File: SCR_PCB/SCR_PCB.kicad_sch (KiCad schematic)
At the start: 4 parts, among them J1 RJ45, J2 Conn_01x03, U2 NA555D, U3 MAX941xSA

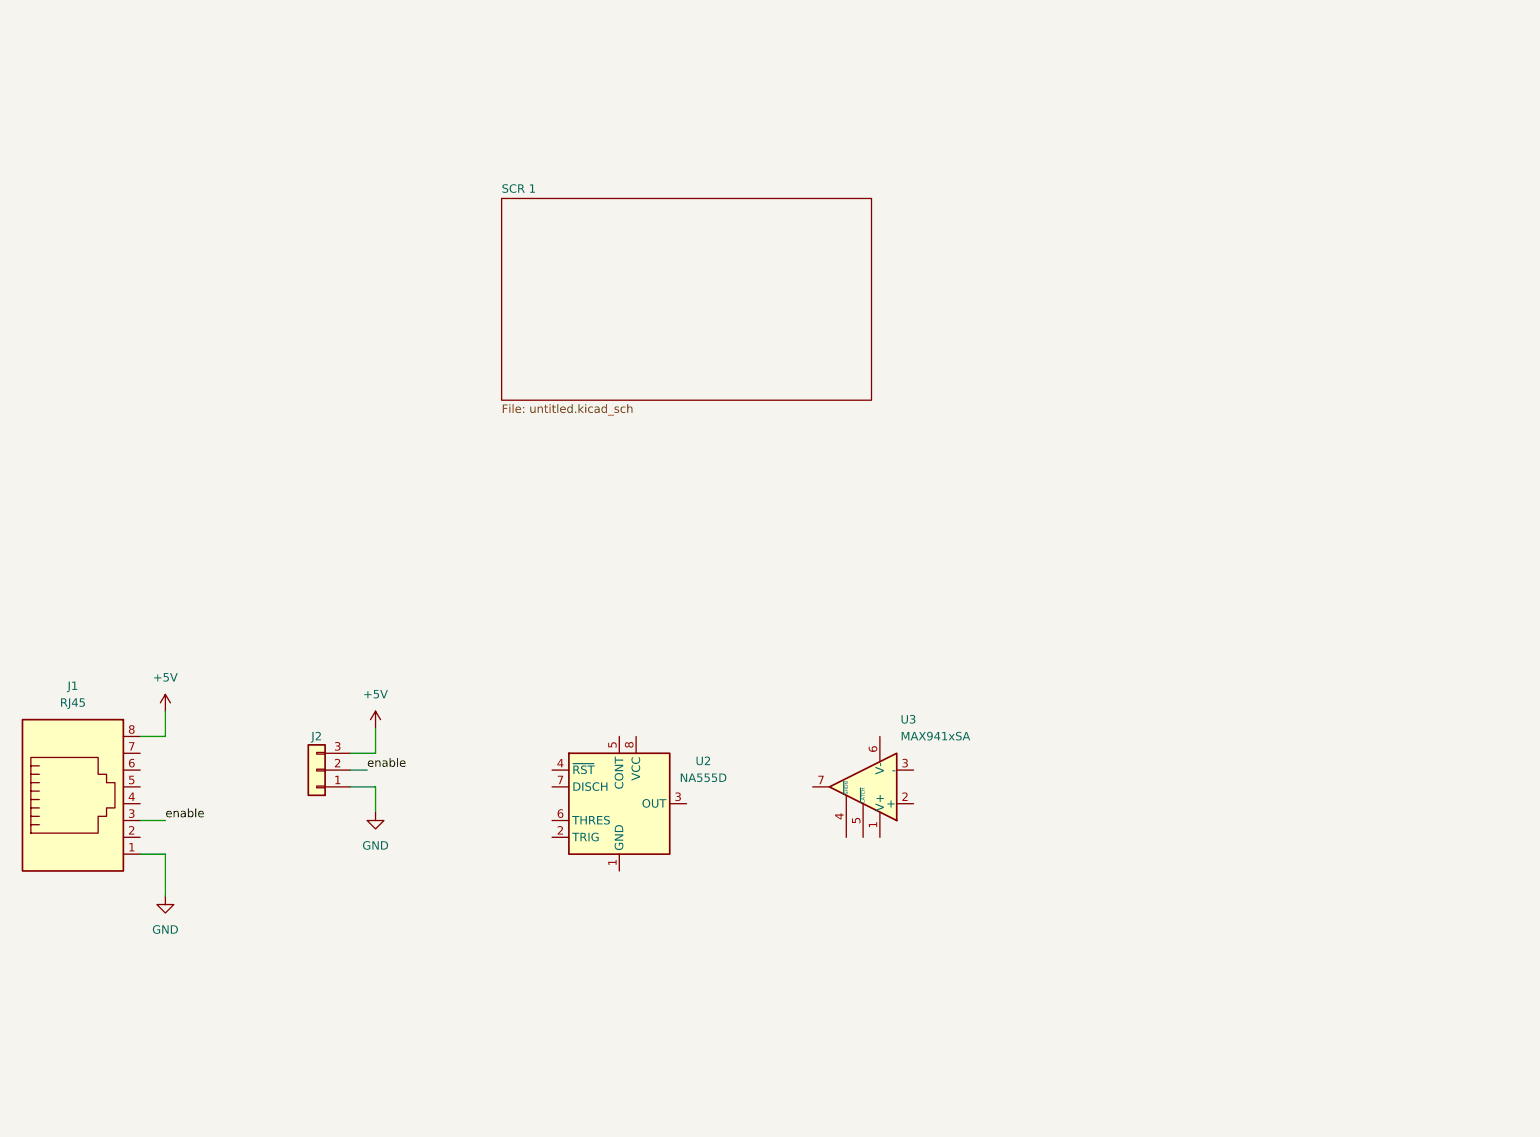
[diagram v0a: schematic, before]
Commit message: update SRC_PCB
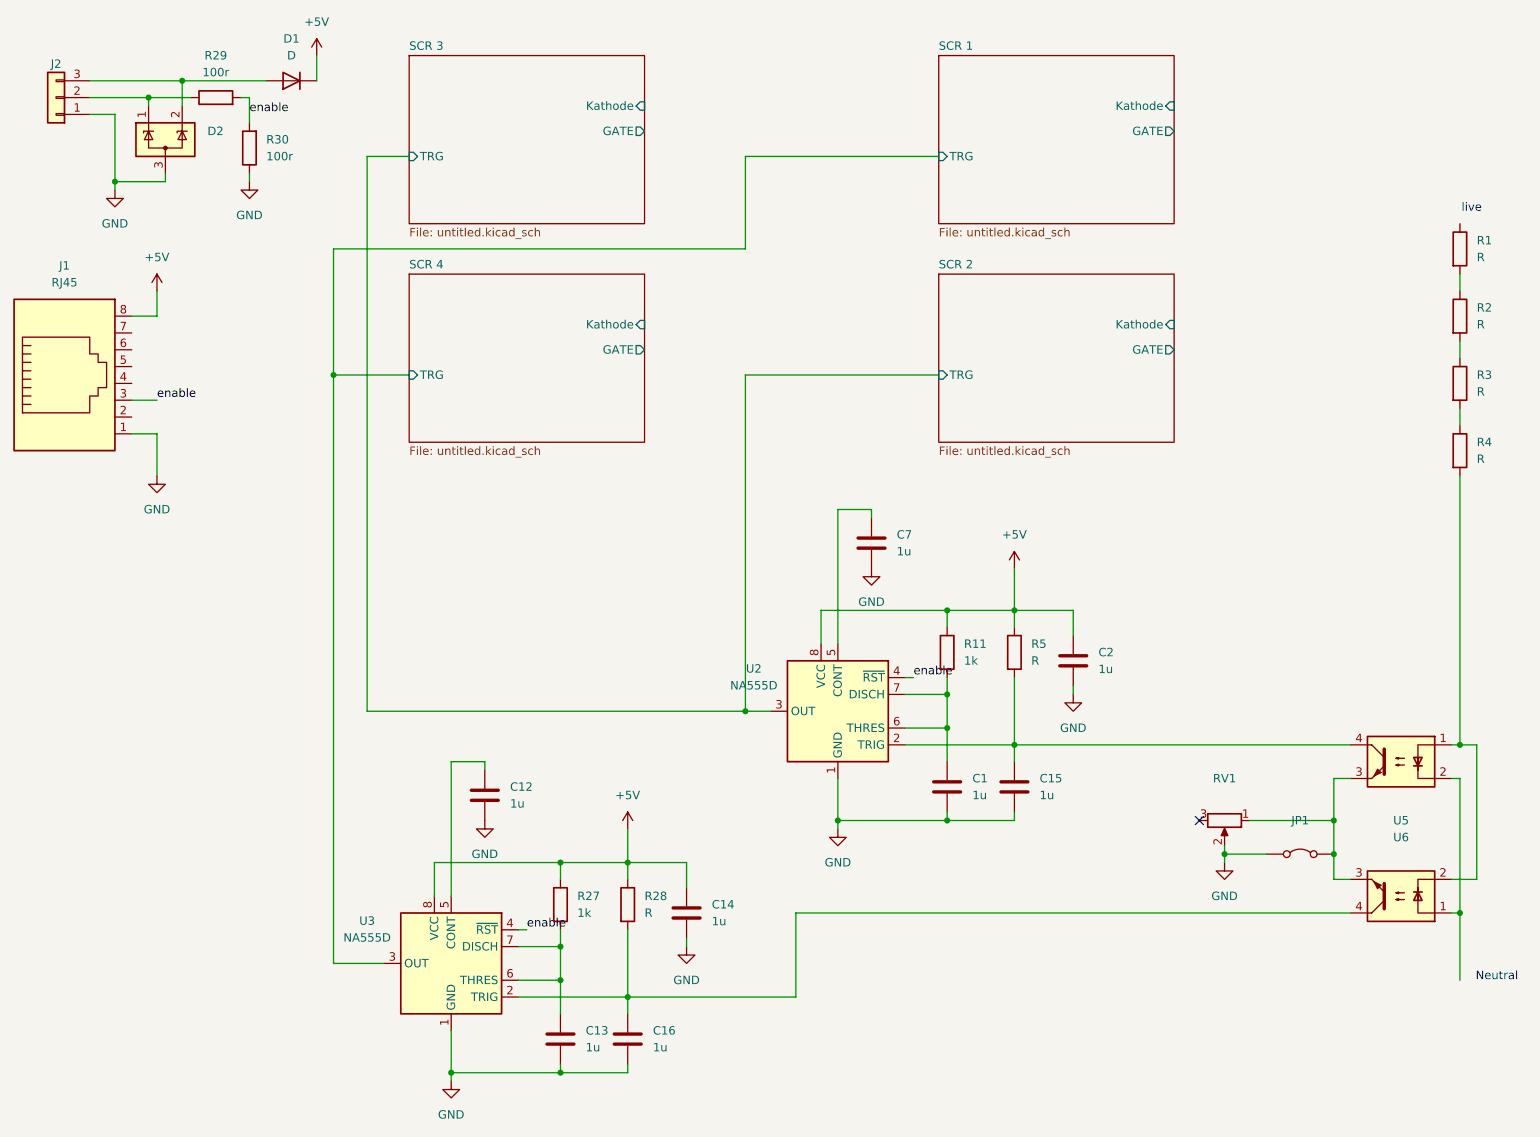
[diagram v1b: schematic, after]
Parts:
- removed U3: MAX941xSA, Package_SO:SOIC-8_3.9x4.9mm_P1.27mm, symbol Comparator:MAX941xSA
- added C1, C12, C13, C14, C15, C16, C2, C7: 1u, symbol Device:C
- added D1: D, symbol Device:D
- added D2: SP0502BAHT, Package_TO_SOT_SMD:SOT-23, symbol Power_Protection:SP0502BAHT
- added JP1: Jumper_2_Bridged, symbol Jumper:Jumper_2_Bridged
- added R1, R2, R28, R3, R4, R5: R, symbol Device:R
- added R11, R27: 1k, symbol Device:R
- added R29, R30: 100r, symbol Device:R
- added RV1: R_Potentiometer, symbol Device:R_Potentiometer
- added U3: NA555D, Package_SO:SOIC-8_3.9x4.9mm_P1.27mm, symbol Timer:NA555D
- added U5, U6: SFH617A-1, Package_DIP:DIP-4_W7.62mm, symbol Isolator:SFH617A-1
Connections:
- net +5V: now also U2.8 (VCC), C14.1, C2.1, D1.1 (K), R11.1, R27.1, R28.1, R5.1, U3.8 (VCC); no longer J2.3 (Pin_3)
- net GND: now also U2.1 (GND), C1.2, C12.2, C13.2, C14.2, C15.2, C16.2, C2.2, C7.2, D2.3 (A), JP1.1 (A), R30.1, RV1.2, U3.1 (GND)
- net enable: now also U2.4 (~{RST}), R29.2, R30.2, U3.4 (~{RST}); no longer J2.2 (Pin_2)
- net at U2.2 (TRIG): now also C15.1, R5.2, U5.4
- net SCR 2/TRG: now reaches U2.3 (OUT)
- net at U2.5 (CONT): now also C7.1
- net at U2.6 (THRES): now also U2.7 (DISCH), C1.1, R11.2
- new net: JP1.2 (B), RV1.1, U5.3, U6.3
- new net: D2.1 (K), J2.2 (Pin_2), R29.1
- new net: D1.2 (A), D2.2 (K), J2.3 (Pin_3)
- new net: R3.2, R4.1
- new net: R4.2, U5.1, U6.2
- new net: R1.2, R2.1
- new net: R2.2, R3.1
- new net: C12.1, U3.5 (CONT)
- new net: C16.1, R28.2, U3.2 (TRIG), U6.4
- new net: C13.1, R27.2, U3.6 (THRES), U3.7 (DISCH)
- new net: U5.2, U6.1
- new net SCR 1/TRG: U3.3 (OUT)
- no-connect marks 0 -> 1
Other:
- added sheet SCR 2 (untitled.kicad_sch)
- added sheet SCR 3 (untitled.kicad_sch)
- added sheet SCR 4 (untitled.kicad_sch)
- sheet SCR 1 ports: added GATE, Kathode, TRG; removed none
- note added: "Neutral"
- note added: "live"
- moved on the sheet: J1, J2, U2
